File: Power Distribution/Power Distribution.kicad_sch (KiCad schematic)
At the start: 12 parts, among them P1 Charging/BoostConverterBoardT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, SW1 SW_Push, U1 Raspberry Pi Zero 2 W, U5 IMU BNO55

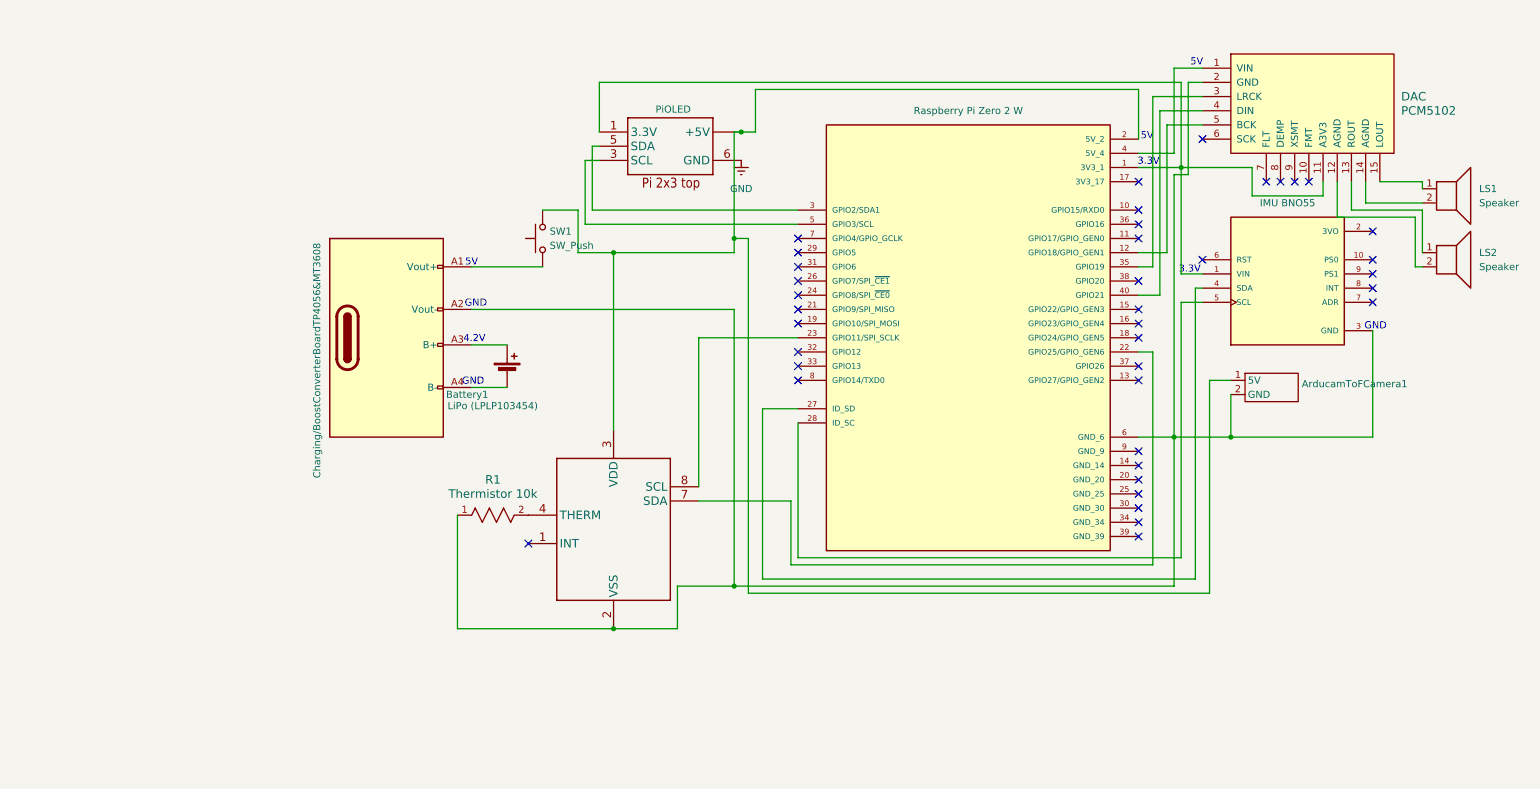
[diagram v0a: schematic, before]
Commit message: updated schematic and PCB
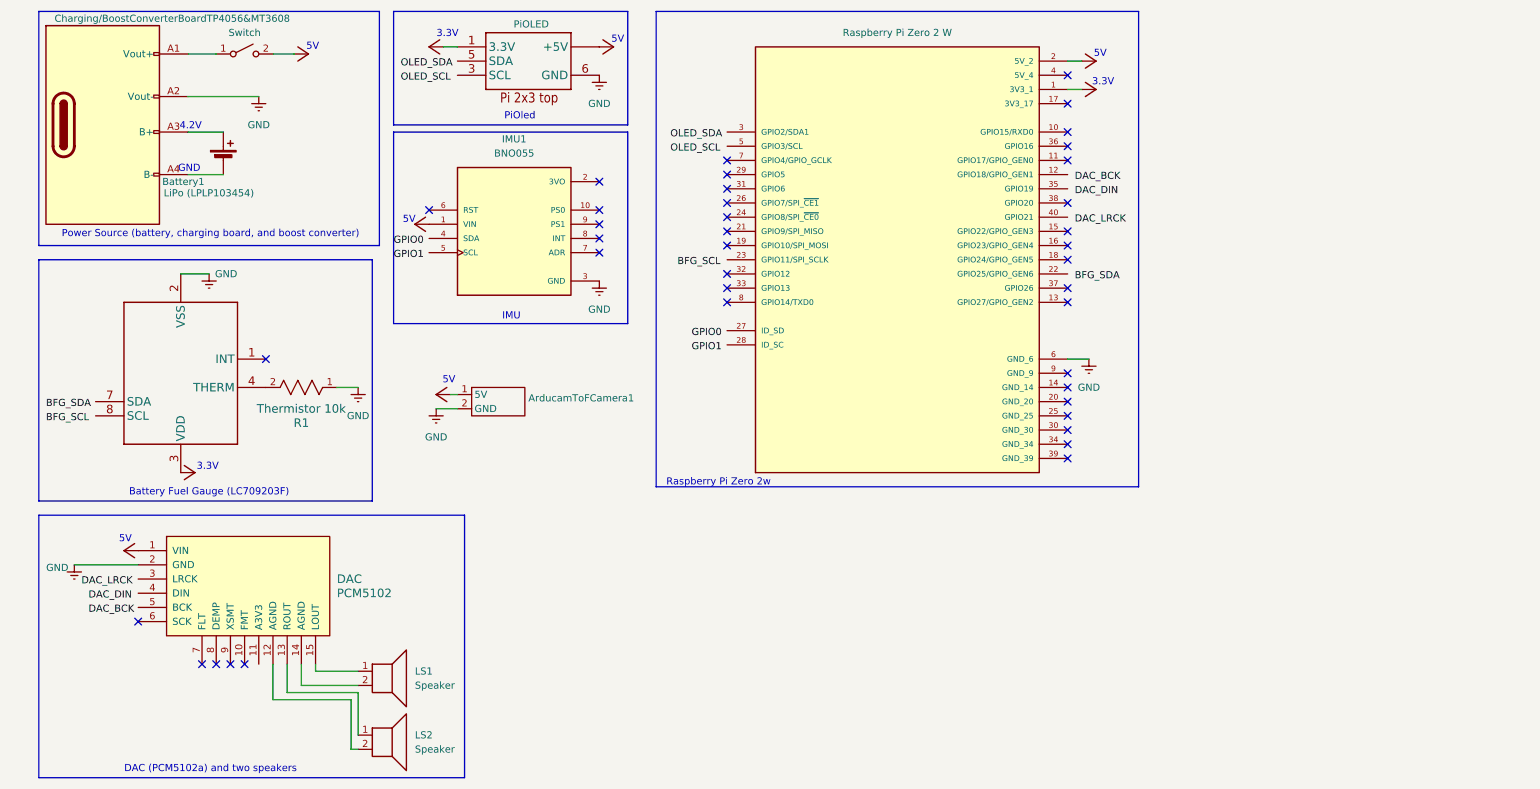
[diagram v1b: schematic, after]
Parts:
- removed SW1: SW_Push, symbol Switch:SW_Push
- removed U5: IMU BNO55, 2472:MODULE_2472, symbol 2472:2472
- added IMU1: BNO055, IMU:MODULE_2472, symbol 2472:2472
- added SW1: Switch, symbol Switch:SW_DPST_x2
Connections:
- net GND: now also 1.2 (VSS), ArducamToFCamera1.2 (GND), DAC.2 (GND), P1.A2 (Vout-), R1.1, U1.6 (GND_6), IMU1.3 (GND)
- net at 1.7 (SDA): no longer U1.22 (GPIO25/GPIO_GEN6)
- net at 1.8 (SCL): no longer U1.23 (GPIO11/SPI_SCLK)
- net at P1.A1 (Vout+), P1.A9 (VBUS), P1.B4 (VBUS)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: now also SW1.1 (A)
- net at PiOLED.3 (SCL): no longer U1.5 (GPIO3/SCL)
- net at PiOLED.5 (SDA): no longer U1.3 (GPIO2/SDA1)
- net at U1.12 (GPIO18/GPIO_GEN1): no longer DAC.5 (BCK)
- net at U1.35 (GPIO19): no longer DAC.3 (LRCK)
- net at U1.4 (5V_4): no longer DAC.1 (VIN)
- net at U1.40 (GPIO21): no longer DAC.4 (DIN)
- new net: PiOLED.2 (+5V), PiOLED.4 (+5V)
- now unconnected: 1.3 (VDD), ArducamToFCamera1.1 (5V), DAC.11 (A3V3), PiOLED.1 (3.3V), U1.1 (3V3_1), U1.2 (5V_2)
- no-connect marks 39 -> 40
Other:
- note added: "Battery Fuel Gauge (LC709203F)"
- note added: "DAC (PCM5102a) and two speakers"
- note added: "IMU"
- note added: "PiOled"
- note added: "Power Source (battery, charging board, and boost converter)"
- note added: "Raspberry Pi Zero 2w"
- moved on the sheet: ArducamToFCamera1, Battery1, DAC, LS1, LS2, PiOLED, R1
